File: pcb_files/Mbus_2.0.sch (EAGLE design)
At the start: 46 parts, among them IC1 NCP1117ST50T3G, IC4 RTC_PCF8523T, J1 F-1X18-SIP-100-32Y, J2 USB_A_SMT_FEMALE, Q1 BSS138, Q2 32.768, Q3 BSS138, Q4 CSM-7X-DU, T1 2N3904, U1 ATMEGA328P-AU

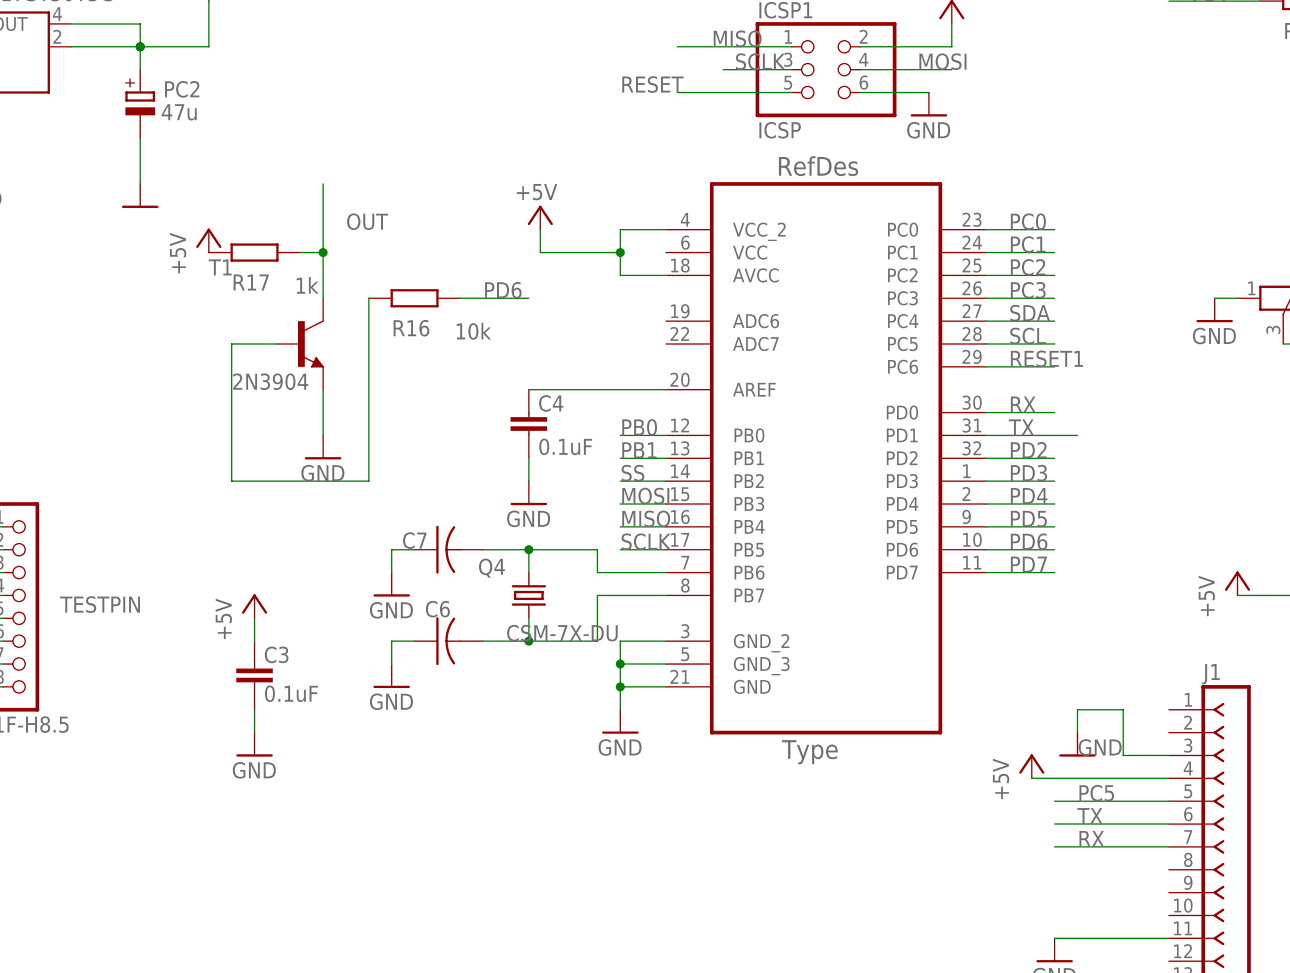
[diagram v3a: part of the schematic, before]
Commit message: pcb 2.0
Signed-off-by: Yiteng Cai <alonsochate@umich.edu>
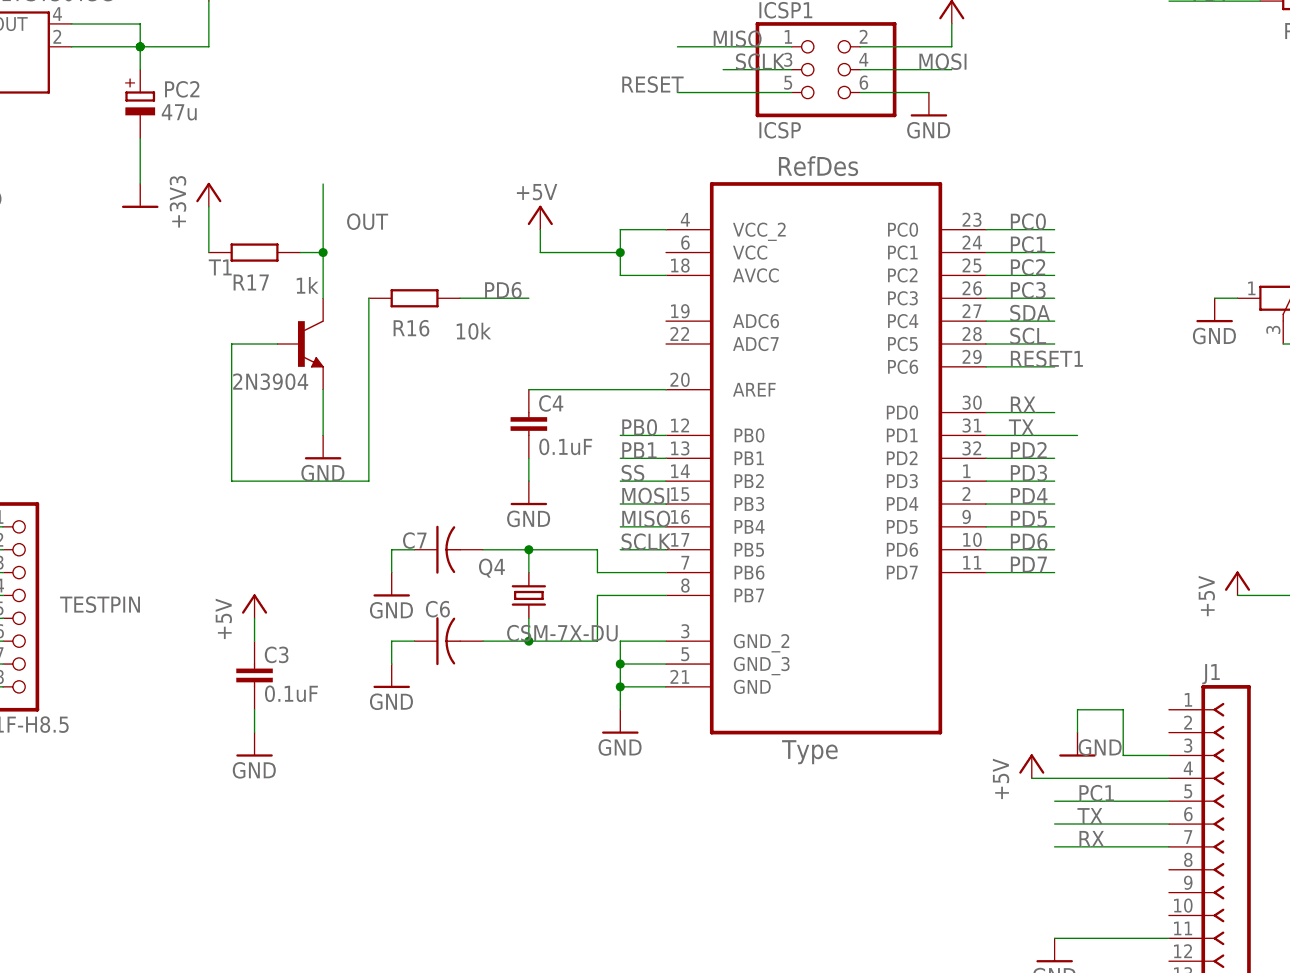
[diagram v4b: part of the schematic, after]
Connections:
- removed net PC5: J1.5
- net +3V3: now also R17.2
- net +5V: no longer R17.2
- net PC1: now also J1.5
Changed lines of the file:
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@@
 <part name="R16" library="SmartPrj" deviceset="R-EU_" device="R0603" value="10k"/>
 <part name="R17" library="SmartPrj" deviceset="R-EU_" device="R0603" value="1k"/>
-<part name="P+15" library="supply1" library_urn="urn:adsk.eagle:library:371" deviceset="+5V" device=""/>
 <part name="GND12" library="supply1" library_urn="urn:adsk.eagle:library:371" deviceset="GND" device=""/>
 <part name="T1" library="transistor" library_urn="urn:adsk.eagle:library:402" deviceset="2N3904" device="" package3d_urn="urn:adsk.eagle:package:28523/2"/>
 <part name="C7" library="rcl" deviceset="C-US" device="C0805"/>
 <part name="POWER" library="pinhead" library_urn="urn:adsk.eagle:library:325" deviceset="PINHD-1X3" device="" package3d_urn="urn:adsk.eagle:package:22458/2"/>
+<part name="+3V6" library="supply1" deviceset="+3V3" device=""/>
 </parts>
 <sheets>
@@
 <attribute name="VALUE" x="98.425" y="97.028" size="1.778" layer="96"/>
 </instance>
-<instance part="P+15" gate="1" x="88.9" y="104.14" smashed="yes">
-<attribute name="VALUE" x="86.36" y="99.06" size="1.778" layer="96" rot="R90"/>
-</instance>
 <instance part="GND12" gate="1" x="101.6" y="78.74" smashed="yes">
 <attribute name="VALUE" x="99.06" y="76.2" size="1.778" layer="96"/>
@@
 <attribute name="NAME" x="13.97" y="64.135" size="1.778" layer="95"/>
 <attribute name="VALUE" x="13.97" y="50.8" size="1.778" layer="96"/>
+</instance>
+<instance part="+3V6" gate="G$1" x="88.9" y="109.22" smashed="yes">
+<attribute name="VALUE" x="86.36" y="104.14" size="1.778" layer="96" rot="R90"/>
 </instance>
 </instances>
@@
 </segment>
 <segment>
-<pinref part="R17" gate="G$1" pin="2"/>
-<pinref part="P+15" gate="1" pin="+5V"/>
-</segment>
-<segment>
 <pinref part="POWER" gate="A" pin="2"/>
 <wire x1="17.78" y1="58.42" x2="7.62" y2="58.42" width="0.1524" layer="91"/>
@@
 <label x="177.8" y="101.6" size="1.778" layer="95"/>
 </segment>
+<segment>
+<wire x1="195.58" y1="40.64" x2="182.88" y2="40.64" width="0.1524" layer="91"/>
+<label x="185.42" y="40.64" size="1.778" layer="95"/>
+<pinref part="J1" gate="G$1" pin="5"/>
+</segment>
 </net>
 <net name="PC2" class="0">
@@
 <wire x1="254" y1="124.46" x2="271.78" y2="124.46" width="0.1524" layer="91"/>
 <wire x1="271.78" y1="124.46" x2="271.78" y2="127" width="0.1524" layer="91"/>
+</segment>
+<segment>
+<pinref part="+3V6" gate="G$1" pin="+3V3"/>
+<pinref part="R17" gate="G$1" pin="2"/>
+<wire x1="88.9" y1="106.68" x2="88.9" y2="101.6" width="0.1524" layer="91"/>
 </segment>
 </net>
@@
 </segment>
 </net>
-<net name="PC5" class="0">
-<segment>
-<wire x1="195.58" y1="40.64" x2="182.88" y2="40.64" width="0.1524" layer="91"/>
-<label x="185.42" y="40.64" size="1.778" layer="95"/>
-<pinref part="J1" gate="G$1" pin="5"/>
-</segment>
-</net>
